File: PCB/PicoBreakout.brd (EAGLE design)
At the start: 88.9 x 57.1 mm, 43 parts

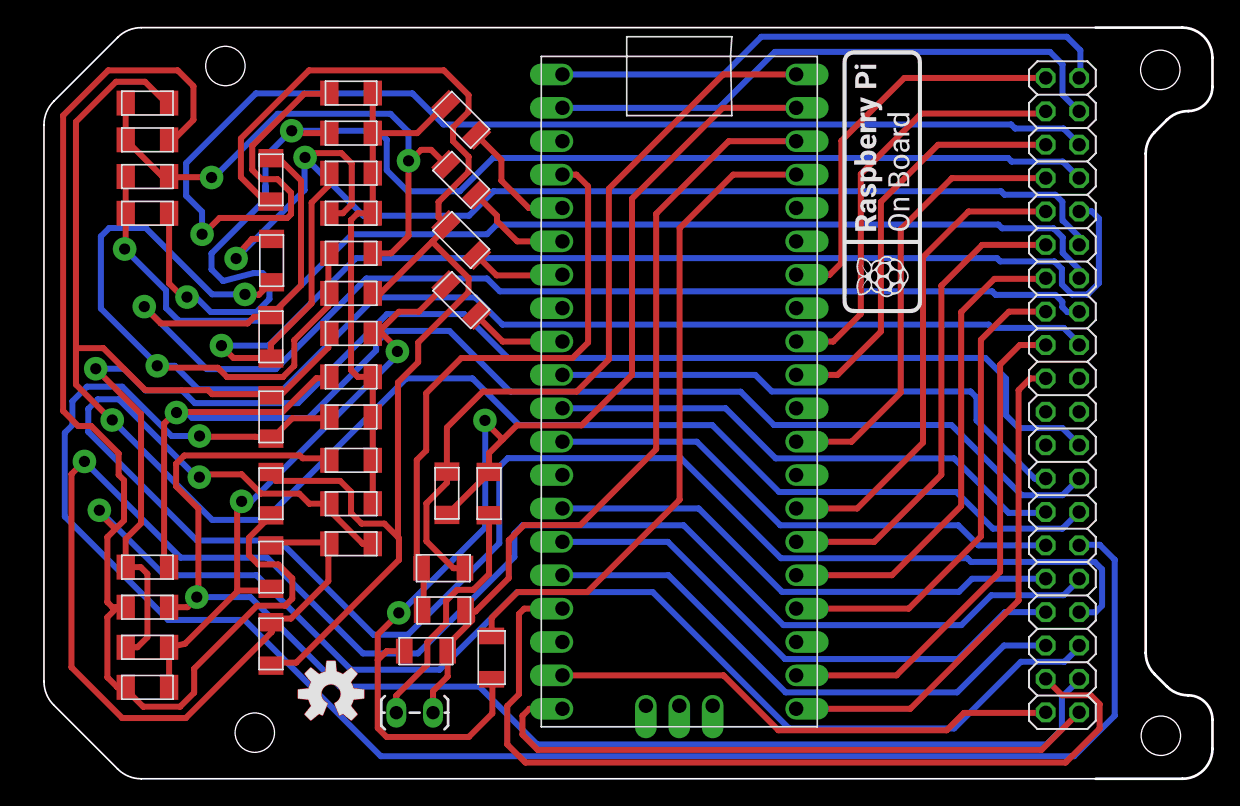
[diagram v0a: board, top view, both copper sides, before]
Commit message: brd updates
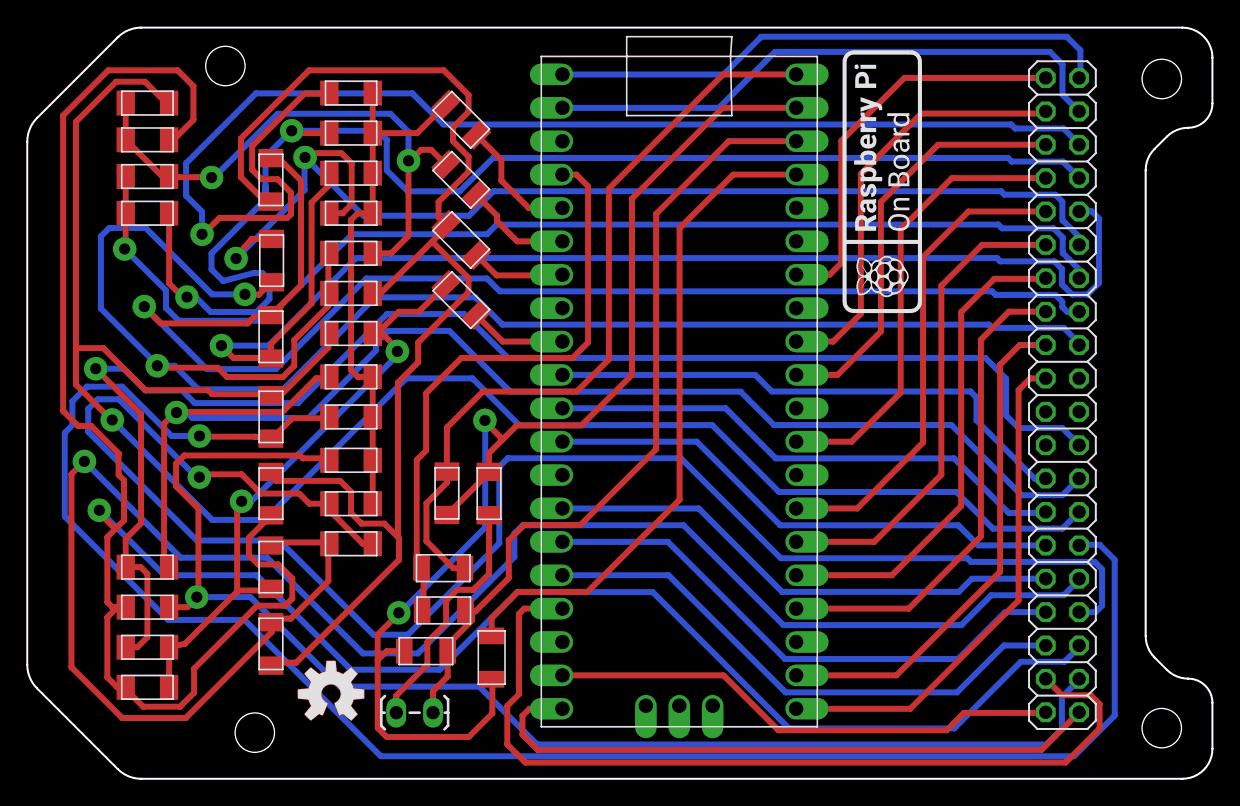
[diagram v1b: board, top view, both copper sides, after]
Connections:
- new net N$64: JP1.20, X1.RUN
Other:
- board size 88.9 x 57.1 mm -> 90.2 x 57.1 mm
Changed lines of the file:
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@@
 <layer number="21" name="tPlace" color="7" fill="1" visible="yes" active="yes"/>
 <layer number="22" name="bPlace" color="7" fill="1" visible="yes" active="yes"/>
-<layer number="23" name="tOrigins" color="15" fill="1" visible="yes" active="yes"/>
-<layer number="24" name="bOrigins" color="15" fill="1" visible="yes" active="yes"/>
+<layer number="23" name="tOrigins" color="15" fill="1" visible="no" active="yes"/>
+<layer number="24" name="bOrigins" color="15" fill="1" visible="no" active="yes"/>
 <layer number="25" name="tNames" color="7" fill="1" visible="yes" active="yes"/>
 <layer number="26" name="bNames" color="7" fill="1" visible="yes" active="yes"/>
@@
 <layer number="45" name="Holes" color="7" fill="1" visible="yes" active="yes"/>
 <layer number="46" name="Milling" color="3" fill="1" visible="no" active="yes"/>
-<layer number="47" name="Measures" color="7" fill="1" visible="yes" active="yes"/>
+<layer number="47" name="Measures" color="7" fill="1" visible="no" active="yes"/>
 <layer number="48" name="Document" color="7" fill="1" visible="no" active="yes"/>
-<layer number="49" name="Reference" color="7" fill="1" visible="yes" active="yes"/>
+<layer number="49" name="Reference" color="7" fill="1" visible="no" active="yes"/>
 <layer number="50" name="dxf" color="7" fill="1" visible="no" active="no"/>
-<layer number="51" name="tDocu" color="7" fill="1" visible="yes" active="yes"/>
-<layer number="52" name="bDocu" color="7" fill="1" visible="yes" active="yes"/>
+<layer number="51" name="tDocu" color="7" fill="1" visible="no" active="yes"/>
+<layer number="52" name="bDocu" color="7" fill="1" visible="no" active="yes"/>
 <layer number="53" name="tGND_GNDA" color="7" fill="9" visible="no" active="no"/>
 <layer number="54" name="bGND_GNDA" color="1" fill="9" visible="no" active="no"/>
@@
 <layer number="128" name="_bValues" color="7" fill="1" visible="no" active="no"/>
 <layer number="129" name="Mask" color="7" fill="1" visible="no" active="no"/>
-<layer number="130" name="SMDSTROOK" color="7" fill="1" visible="yes" active="yes"/>
+<layer number="130" name="SMDSTROOK" color="7" fill="1" visible="no" active="yes"/>
 <layer number="131" name="tAdjust" color="7" fill="1" visible="no" active="no"/>
 <layer number="132" name="bAdjust" color="7" fill="1" visible="no" active="no"/>
 <layer number="133" name="133bmp" color="1" fill="10" visible="no" active="yes"/>
 <layer number="134" name="silk_top" color="7" fill="1" visible="no" active="no"/>
-<layer number="135" name="silk_bottom" color="7" fill="1" visible="yes" active="yes"/>
+<layer number="135" name="silk_bottom" color="7" fill="1" visible="no" active="yes"/>
 <layer number="136" name="silktop" color="7" fill="1" visible="no" active="no"/>
 <layer number="137" name="silkbottom" color="7" fill="1" visible="no" active="no"/>
@@
 <layer number="196" name="mValues" color="7" fill="1" visible="no" active="no"/>
 <layer number="199" name="Contour" color="7" fill="1" visible="no" active="no"/>
-<layer number="200" name="200bmp" color="1" fill="10" visible="yes" active="yes"/>
+<layer number="200" name="200bmp" color="1" fill="10" visible="no" active="yes"/>
 <layer number="201" name="201bmp" color="2" fill="10" visible="no" active="no"/>
 <layer number="202" name="202bmp" color="3" fill="10" visible="no" active="no"/>
@@
 </layers>
 <board>
-<fusionsync huburn="a.cGVyc29uYWw6dWUyY2VjZDkz" projecturn="a.cGVyc29uYWw6dWUyY2VjZDkzIzIwMTkwMTAzMTY4MjEzNTA2" f3durn="urn:adsk.wipprod:dm.lineage:g2FzlmCfS4iXO2IOv7ZSYg" pcbguid="89c8c0a1-dd69-4ef4-b93a-1f64f55537e1" lastpulledtime="" lastsyncedchangeguid="" latestrevisionid="3ed4198d-4a7d-471d-a0de-3c94c9aa8158" lastsyncedrevisionid="3ed4198d-4a7d-471d-a0de-3c94c9aa8158" lastboardhashguid="849b84f2-fd19-473c-12fe-b8a419a203dc" lastpushedtime="2023-01-17T13:23:22Z" linktopcb3d="true"/>
+<fusionsync huburn="a.cGVyc29uYWw6dWUyY2VjZDkz" projecturn="a.cGVyc29uYWw6dWUyY2VjZDkzIzIwMTkwMTAzMTY4MjEzNTA2" f3durn="urn:adsk.wipprod:dm.lineage:ixqSRqazQ6iq9kh7N2QCNw" pcbguid="" lastpulledtime="" lastsyncedchangeguid="" latestrevisionid="6787409e-c346-474f-86f8-f629485dc88d" lastsyncedrevisionid="6787409e-c346-474f-86f8-f629485dc88d" lastboardhashguid="dbcc62ec-450a-83ad-d352-66f7236cc833" lastpushedtime="2023-01-18T13:37:16Z" linktopcb3d="false"/>
 <plain>
 <text x="37.587415625" y="7.9738875" size="1.016" layer="27" rot="R90">100k</text>
 <text x="30.24874375" y="2.30908125" size="2" layer="27" font="vector">-</text>
 <text x="27.383096875" y="2.30908125" size="2" layer="27" font="vector">+</text>
-<wire x1="81.28" y1="57.15" x2="8.672103125" y2="57.15" width="0.127" layer="20"/>
-<wire x1="8.672103125" y1="57.15" x2="6.87605" y2="56.40605" width="0.127" layer="20" curve="45.00005"/>
-<wire x1="6.87605" y1="56.40605" x2="2.01395" y2="51.54395" width="0.127" layer="20"/>
-<wire x1="2.01395" y1="51.54395" x2="1.27" y2="49.747896875" width="0.127" layer="20" curve="45.00007"/>
-<wire x1="1.27" y1="49.747896875" x2="1.27" y2="7.402103125" width="0.127" layer="20"/>
-<wire x1="1.27" y1="7.402103125" x2="2.01395" y2="5.60605" width="0.127" layer="20" curve="45.00005"/>
-<wire x1="2.01395" y1="5.60605" x2="6.87605" y2="0.74395" width="0.127" layer="20"/>
-<wire x1="6.87605" y1="0.74395" x2="8.672103125" y2="0" width="0.127" layer="20" curve="45.00007"/>
-<wire x1="8.672103125" y1="0" x2="81.28" y2="0" width="0.127" layer="20"/>
 <hole x="15.071340625" y="54.229565625" drill="3"/>
 <hole x="17.30965625" y="3.510728125" drill="3"/>
-<hole x="86.20316875" y="53.934209375" drill="3"/>
-<hole x="86.24433125" y="3.274575" drill="3"/>
-<wire x1="81.28" y1="0" x2="87.884" y2="0" width="0.2032" layer="20"/>
-<wire x1="87.884" y1="0" x2="90.17" y2="2.286" width="0.2032" layer="20" curve="90"/>
-<wire x1="90.17" y1="2.286" x2="90.17" y2="4.50289375" width="0.2032" layer="20"/>
-<wire x1="90.17" y1="4.50289375" x2="88.32289375" y2="6.35" width="0.2032" layer="20" curve="90"/>
-<wire x1="88.32289375" y1="6.35" x2="86.706446875" y2="7.019553125" width="0.2032" layer="20" curve="-45"/>
-<wire x1="86.706446875" y1="7.019553125" x2="85.759553125" y2="7.966446875" width="0.2032" layer="20"/>
-<wire x1="85.759553125" y1="7.966446875" x2="85.09" y2="9.58289375" width="0.2032" layer="20" curve="-45"/>
-<wire x1="85.09" y1="9.58289375" x2="85.09" y2="47.56710625" width="0.2032" layer="20"/>
-<wire x1="85.09" y1="47.56710625" x2="85.759553125" y2="49.183553125" width="0.2032" layer="20" curve="-45"/>
-<wire x1="85.759553125" y1="49.183553125" x2="86.706446875" y2="50.130446875" width="0.2032" layer="20"/>
-<wire x1="86.706446875" y1="50.130446875" x2="88.32289375" y2="50.8" width="0.2032" layer="20" curve="-45"/>
-<wire x1="88.32289375" y1="50.8" x2="90.17" y2="52.64710625" width="0.2032" layer="20" curve="90"/>
-<wire x1="90.17" y1="52.64710625" x2="90.17" y2="54.864" width="0.2032" layer="20"/>
-<wire x1="90.17" y1="54.864" x2="87.884" y2="57.15" width="0.2032" layer="20" curve="90"/>
-<wire x1="87.884" y1="57.15" x2="81.28" y2="57.15" width="0.2032" layer="20"/>
+<hole x="86.317740625" y="53.242246875" drill="3"/>
+<hole x="86.3155625" y="3.852196875" drill="3"/>
+<wire x1="87.884" y1="0" x2="8.672103125" y2="0" width="0.1524" layer="20"/>
+<wire x1="8.672103125" y1="0" x2="6.87605" y2="0.74395" width="0.1524" layer="20" curve="-45.00005"/>
+<wire x1="6.87605" y1="0.74395" x2="0.74395" y2="6.87605" width="0.1524" layer="20"/>
+<wire x1="0.74395" y1="6.87605" x2="0" y2="8.672103125" width="0.1524" layer="20" curve="-45.00007"/>
+<wire x1="0" y1="8.672103125" x2="0" y2="48.477896875" width="0.1524" layer="20"/>
+<wire x1="0" y1="48.477896875" x2="0.74395" y2="50.27395" width="0.1524" layer="20" curve="-45.00005"/>
+<wire x1="0.74395" y1="50.27395" x2="6.87605" y2="56.40605" width="0.1524" layer="20"/>
+<wire x1="6.87605" y1="56.40605" x2="8.672103125" y2="57.15" width="0.1524" layer="20" curve="-45.00007"/>
+<wire x1="8.672103125" y1="57.15" x2="87.884" y2="57.15" width="0.1524" layer="20"/>
+<wire x1="87.884" y1="57.15" x2="90.17" y2="54.864" width="0.1524" layer="20" curve="-90"/>
+<wire x1="90.17" y1="54.864" x2="90.17" y2="51.37710625" width="0.1524" layer="20"/>
+<wire x1="90.17" y1="51.37710625" x2="88.32289375" y2="49.53" width="0.1524" layer="20" curve="-90"/>
+<wire x1="88.32289375" y1="49.53" x2="86.706446875" y2="48.860446875" width="0.1524" layer="20" curve="45"/>
+<wire x1="86.706446875" y1="48.860446875" x2="85.759553125" y2="47.913553125" width="0.1524" layer="20"/>
+<wire x1="85.759553125" y1="47.913553125" x2="85.09" y2="46.29710625" width="0.1524" layer="20" curve="45"/>
+<wire x1="85.09" y1="46.29710625" x2="85.09" y2="10.85289375" width="0.1524" layer="20"/>
+<wire x1="85.09" y1="10.85289375" x2="85.759553125" y2="9.236446875" width="0.1524" layer="20" curve="45"/>
+<wire x1="85.759553125" y1="9.236446875" x2="86.706446875" y2="8.289553125" width="0.1524" layer="20"/>
+<wire x1="86.706446875" y1="8.289553125" x2="88.32289375" y2="7.62" width="0.1524" layer="20" curve="45"/>
+<wire x1="88.32289375" y1="7.62" x2="90.17" y2="5.77289375" width="0.1524" layer="20" curve="-90"/>
+<wire x1="90.17" y1="5.77289375" x2="90.17" y2="2.286" width="0.1524" layer="20"/>
+<wire x1="90.17" y1="2.286" x2="87.884" y2="0" width="0.1524" layer="20" curve="-90"/>
 </plain>
 <attributes>
@@
 <wire x1="75.59078125" y1="8.902146875" x2="78.912853125" y2="8.902146875" width="0.4572" layer="16"/>
 </signal>
+<signal name="N$64">
+<contactref element="JP1" pad="20"/>
+<contactref element="X1" pad="RUN"/>
+<wire x1="58.495415625" y1="28.1868875" x2="80.025671875" y2="30.45934375" width="0" layer="19" extent="1-1"/>
+</signal>
 </signals>
